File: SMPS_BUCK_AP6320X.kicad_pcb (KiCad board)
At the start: 2 copper layers, 14.4 x 14.6 mm, 12 parts, among them U2 AP63205WU-7

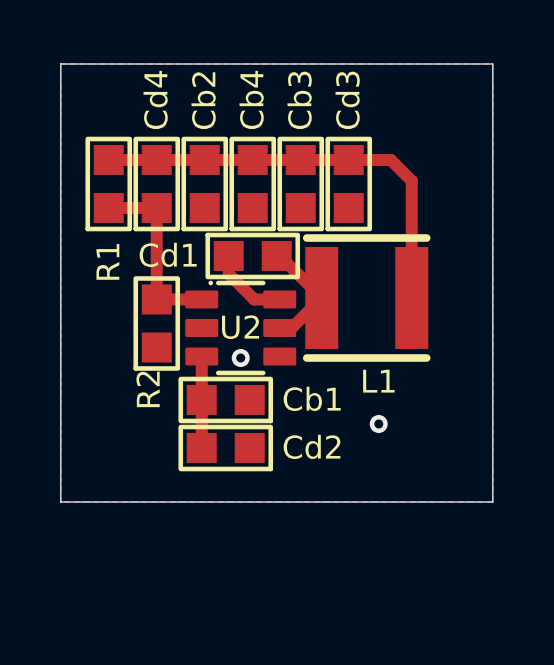
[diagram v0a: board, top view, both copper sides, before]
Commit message: New layout.
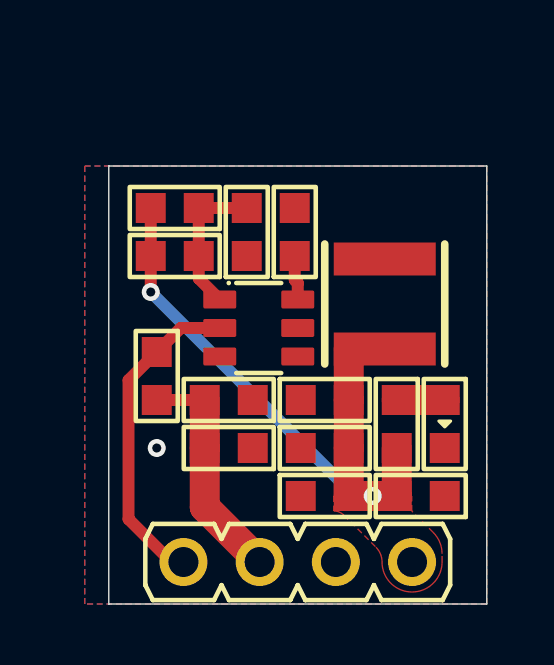
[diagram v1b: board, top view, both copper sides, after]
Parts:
- added D1: LTST-C190KFKT, kicad_lib:Lite-On_LTST-C190KFKT, F.Cu at (159.2, 118.2)
- added J1: 61300411121, kicad_lib:Würth_Elektronik_61300411121, B.Cu at (154.3, 122.8)
- added R3: 10 kΩ, kicad_lib:YAGEO_RC0603FR-070RL, F.Cu at (157.6, 118.2)
- added R4: 10 kΩ, kicad_lib:YAGEO_RC0603FR-070RL, F.Cu at (149.6, 116.6)
- added REF**: Untitled, kicad_lib:agro_logo_10mm, B.Cu at (155.4, 114.6)
- moved Cb4 11.8 mm to (158.4, 120.6), turned to 180 degrees
- moved Cb2 11.1 mm to (155.2, 120.6), turned to 0 degrees
- moved Cb3 8.84 mm to (155.2, 119.0), turned to 0 degrees
- moved Cd3 7.24 mm to (155.2, 117.4), turned to 0 degrees
- moved R2 4.28 mm to (152.6, 111.8)
- moved R1 3.26 mm to (150.2, 112.6), turned to 180 degrees
- moved Cd1 1.61 mm to (154.2, 111.8), turned to 90 degrees
- moved Cd4 1.00 mm to (150.2, 111.0), turned to 180 degrees
- moved L1 0.63 mm to (157.2, 114.2), turned to 0 degrees
- moved U2 0.60 mm to (153.0, 115.0)
- moved Cb1 0.10 mm to (152.0, 117.4)
- moved Cd2 0.10 mm to (152.0, 119.0)
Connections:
- net /OUT renamed /VOUT
- U2 pad 2: unconnected-(U2-EN-Pad2) -> /EN
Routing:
- net /EN: track 0.00 -> 10.4 mm
- net /VOUT: track 14.3 -> 22.3 mm, vias 0 -> 2
- net /VIN: track 3.05 -> 7.76 mm
- net Net-(U2-SW): track 3.89 -> 0.00 mm
- net Net-(D1-PadA): track 0.00 -> 1.60 mm
- net /FB: track 6.15 -> 4.94 mm
- net Net-(U2-BST): track 2.65 -> 1.49 mm
- net GND: vias 2 -> 1
- added copper zone on F.Cu, net /VOUT
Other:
- board size 14.4 x 14.6 mm -> 12.6 x 14.6 mm
